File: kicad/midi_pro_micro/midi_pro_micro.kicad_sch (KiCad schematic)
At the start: 27 parts, among them J1 DIN-5_180degree, J2 DIN-5_180degree, J4 Conn_01x16_Pin, SW1 RotaryEncoder_Switch, SW6 SW_Push_LEDx5, U1 ProMicro, U2 AT25xxx, U3 6N138

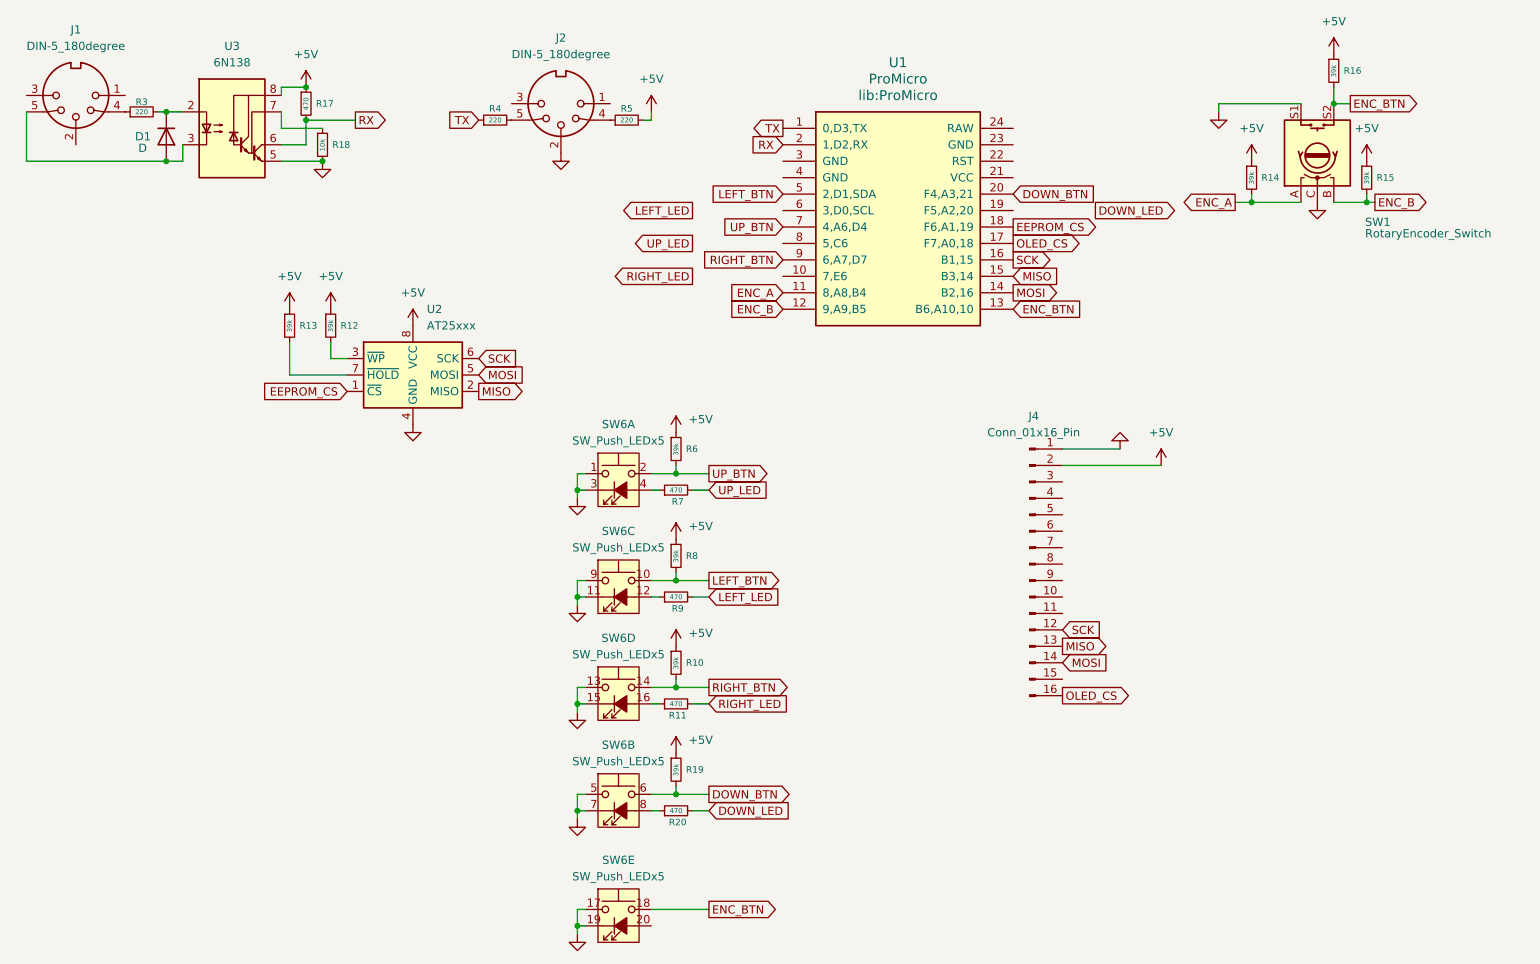
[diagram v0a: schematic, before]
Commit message: 5-way-button board
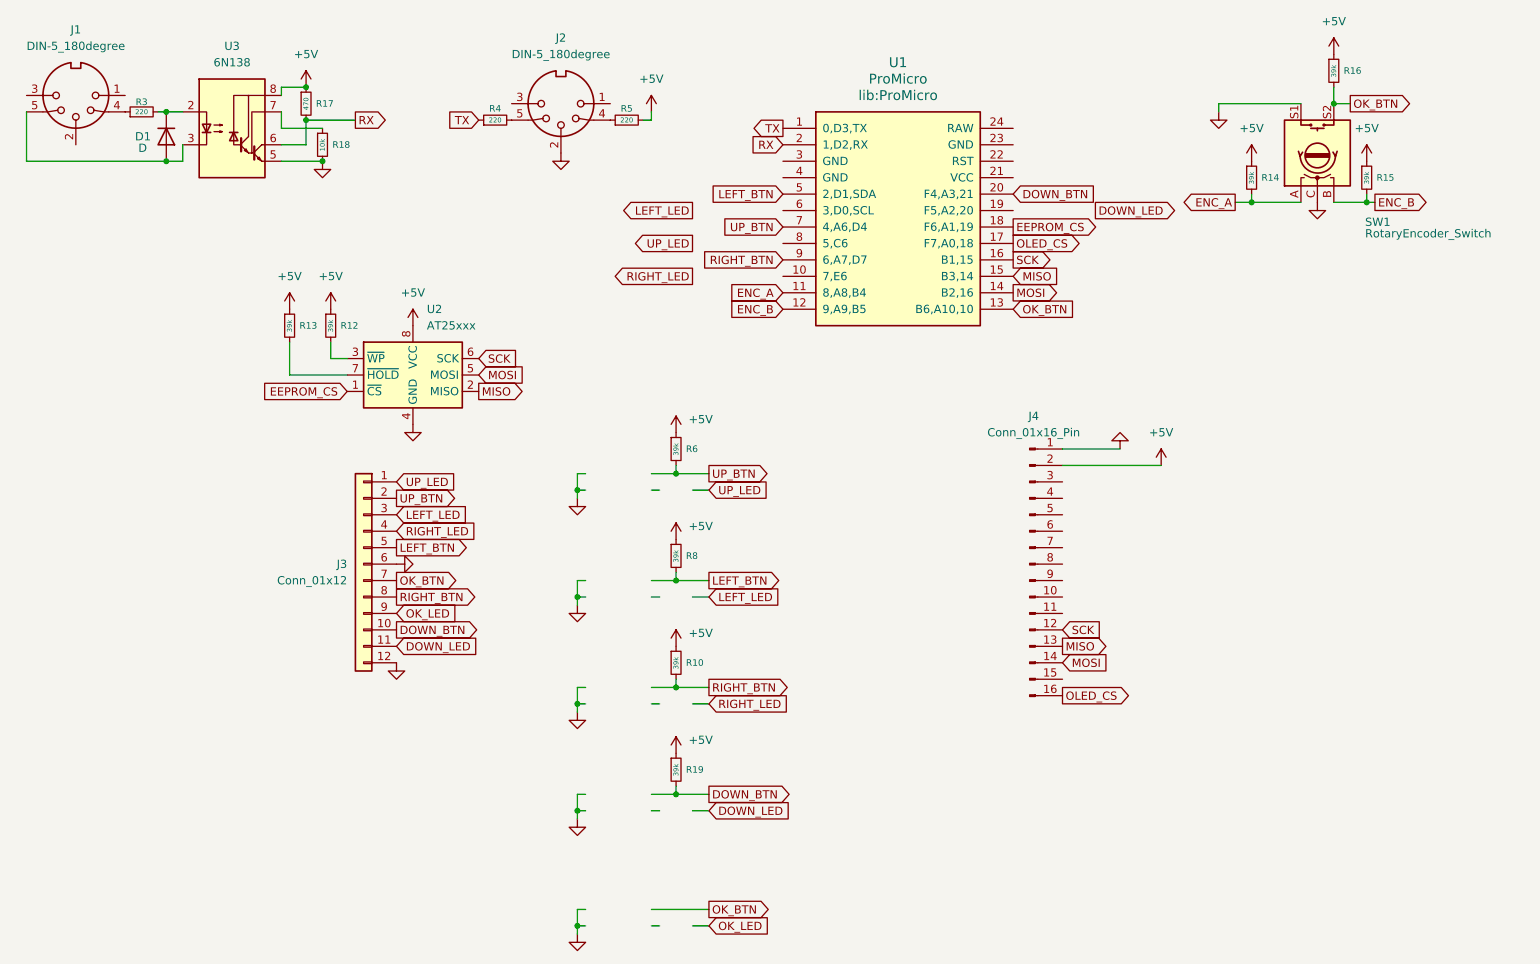
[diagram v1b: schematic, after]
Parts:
- removed R11, R20, R7, R9: 470, Resistor_SMD:R_0805_2012Metric_Pad1.20x1.40mm_HandSolder, symbol Device:R_Small
- removed SW6: SW_Push_LEDx5, lib:SW_PUSH_12mm_LEDx5, symbol 5-way-buttons:SW_Push_LEDx5
- added J3: Conn_01x12, lib:SW_PUSH_12mm_LEDx5_BOARD, symbol Connector_Generic:Conn_01x12
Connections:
- net DOWN_BTN: now also J3.10 (Pin_10)
- net DOWN_LED: now also J3.11 (Pin_11)
- net GND: now also J3.12 (Pin_12), J3.6 (Pin_6)
- net LEFT_BTN: now also J3.5 (Pin_5)
- net LEFT_LED: now also J3.3 (Pin_3)
- net RIGHT_BTN: now also J3.8 (Pin_8)
- net RIGHT_LED: now also J3.4 (Pin_4)
- net UP_BTN: now also J3.2 (Pin_2)
- net UP_LED: now also J3.1 (Pin_1)
- net ENC_BTN renamed OK_BTN
- net OK_BTN: now also J3.7 (Pin_7)
- new net OK_LED: J3.9 (Pin_9)
